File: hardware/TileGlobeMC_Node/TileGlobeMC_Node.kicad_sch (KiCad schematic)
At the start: 112 parts, among them J1 Conn_01x05, J10 LCD, J11 USB_C, J2 P_Male, J3 Conn_01x05, J4 P_Male, J5 Conn_01x05, J6 P_Male, J7 Conn_01x05, J8 P_Male, J9 SWD, Q1 2N7002, Q2 2N7002, SW1 Left, SW2 Left, SW3 Left, SW4 Left, SW5 Left, U1 RP2350_80QFN, U2 TPS62A01DRL, U3 BQ24232RGT, U4 ESP-PSRAM64H, U5 PY25Q128HA-WXH, U6 PY25Q128HA-SSH, U7 74AHC1G04, U8 SC7A20, Y1 12M

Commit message: PCB progress
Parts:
- removed BT1: LIR2032, symbol Device:Battery_Cell
- removed C1, C12, C2, C27, C3, C4, C5, C6, C7, C9: 4.7u, Capacitor_SMD:C_0402_1005Metric, symbol Device:C_Small
- removed C10, C11, C13, C14, C15, C16, C17, C18, C19, C20, C21, C22, C25, C26, C28, C29, C30, C31, C32, C33, C34: 100n, Capacitor_SMD:C_0402_1005Metric, symbol Device:C_Small
- removed C23, C24: 15p, Capacitor_SMD:C_0402_1005Metric, symbol Device:C_Small
- removed C8: 22u, Capacitor_SMD:C_0603_1608Metric, symbol Device:C_Small
- removed D1, D2, D4: 1N4148WT, Diode_SMD:D_SOD-523, symbol Diode:1N4148WT
- removed D3, D5: 3V, Diode_SMD:D_SOD-523, symbol Device:D_Zener_Small
- removed J1, J3, J5, J7: Conn_01x05, symbol Connector_Generic:Conn_01x05
- removed J10: LCD, Connector_FFC-FPC:TE_1-1734839-2_1x12-1MP_P0.5mm_Horizontal, symbol Connector_Generic_MountingPin:Conn_01x12_MountingPin
- removed J11: USB_C, Connector_USB:USB_C_Receptacle_GCT_USB4105-xx-A_16P_TopMnt_Horizontal, symbol Connector:USB_C_Receptacle_USB2.0_16P
- removed J2, J4, J6, J8: P_Male, Project:BC-15-5P380, symbol Connector_Generic_MountingPin:Conn_01x05_MountingPin
- removed J9: SWD, Connector_JST:JST_SH_BM03B-SRSS-TB_1x03-1MP_P1.00mm_Vertical, symbol Connector_Generic_MountingPin:Conn_01x03_MountingPin
- removed JP1: RESET, TestPoint:TestPoint_2Pads_Pitch2.54mm_Drill0.8mm, symbol Jumper:Jumper_2_Small_Open
- removed JP2: USB_BOOT, TestPoint:TestPoint_2Pads_Pitch2.54mm_Drill0.8mm, symbol Jumper:Jumper_2_Small_Open
- removed L1: 3.3u, RP2350:L_pol_2016, symbol Project:L_Polarized_Ferrite_Small
- removed L2: 1u, Inductor_SMD:L_Wuerth_MAPI-2010, symbol Device:L_Ferrite_Small
- removed Q1, Q2: 2N7002, Package_TO_SOT_SMD:SOT-23, symbol Transistor_FET:2N7002
- removed R1, R10, R4, R7: 300, Capacitor_SMD:C_0402_1005Metric, symbol Device:R_Small
- removed R11, R12, R2, R3, R5, R6, R8, R9: 270, Capacitor_SMD:C_0402_1005Metric, symbol Device:R_Small
- removed R13, R24: 33, Capacitor_SMD:C_0402_1005Metric, symbol Device:R_Small
- removed R14, R35, R36, R37, R38, R39, R40, R41: 10k, Capacitor_SMD:C_0402_1005Metric, symbol Device:R_Small
- removed R15: 17.4k, Capacitor_SMD:C_0402_1005Metric, symbol Device:R_Small
- removed R16: 1.5k, Capacitor_SMD:C_0402_1005Metric, symbol Device:R_Small
- removed R17, R18, R19, R22, R23, R28, R29, R34: 100k, Capacitor_SMD:C_0402_1005Metric, symbol Device:R_Small
- removed R20: 86.6k, Capacitor_SMD:C_0402_1005Metric, symbol Device:R_Small
- removed R21: 390k, Capacitor_SMD:C_0402_1005Metric, symbol Device:R_Small
- removed R25, R30: 1k, Capacitor_SMD:C_0402_1005Metric, symbol Device:R_Small
- removed R26, R27: 27, Capacitor_SMD:C_0402_1005Metric, symbol Device:R_Small
- removed R31: 4.7, Capacitor_SMD:C_0402_1005Metric, symbol Device:R_Small
- removed R32, R33: 5.1k, Capacitor_SMD:C_0402_1005Metric, symbol Device:R_Small
- removed SW1, SW2, SW3, SW4, SW5: Left, Button_Switch_SMD:SW_SPST_PTS647_Sx38, symbol Switch:SW_Push
- removed U1: RP2350_80QFN, RP2350:RP2350-QFN-80-1EP_10x10_P0.4mm_EP3.4x3.4mm_ThermalVias, symbol RP2350:RP2350_80QFN
- removed U2: TPS62A01DRL, Package_TO_SOT_SMD:SOT-563, symbol Regulator_Switching:TPS62A01DRL
- removed U3: BQ24232RGT, Package_DFN_QFN:VQFN-16-1EP_3x3mm_P0.5mm_EP1.68x1.68mm_ThermalVias, symbol Project:BQ24232RGT
- removed U4: ESP-PSRAM64H, Package_SO:SOIC-8_3.9x4.9mm_P1.27mm, symbol Project:ESP-PSRAM64
- removed U5: PY25Q128HA-WXH, Package_SON:WSON-8-1EP_6x5mm_P1.27mm_EP3.4x4.3mm, symbol Memory_Flash:W25Q128JVP
- removed U6: PY25Q128HA-SSH, Package_SO:SOIC-8_5.3x5.3mm_P1.27mm, symbol Memory_Flash:W25Q128JVS
- removed U7: 74AHC1G04, Package_TO_SOT_SMD:SOT-23-5, symbol 74xGxx:74AHC1G04
- removed U8: SC7A20, Package_LGA:LGA-12_2x2mm_P0.5mm, symbol Sensor_Motion:SC7A20
- removed Y1: 12M, Crystal:Crystal_SMD_3225-4Pin_3.2x2.5mm, symbol Device:Crystal_GND24
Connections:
- no-connect marks 10 -> 29
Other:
- removed sheet Power
- sheet Core ports: added +3V3, BTN_CENTER, BTN_CENTER_VBUS, GND_CORE, GPIO0, GPIO1, GPIO2, GPIO3, GPIO4, I2C_SCL, I2C_SDA, LCD_CS, LCD_DC, LCD_MOSI, LCD_SCK, PERI_INT, VBUS; removed none
- sheet Peripheral ports: added +3V3, BTN_CENTER, BTN_CENTER_VBUS, GND_PERI, I2C_SCL, I2C_SDA, LCD_CS, LCD_DC, LCD_MOSI, LCD_SCK, PERI_INT, VBUS; removed none
- note removed: "3.3V DC-DC"
- note removed: "Battery Charger & Power Path"
- note removed: "Buttons"
- note removed: "Flash & PSRAM"
- note removed: "IMU"
- note removed: "LCD"
- note removed: "Node Ports"
- note removed: "Note: buttons use MCU's internal pull-down."
- note removed: "TODO: change setting resistors now that we're using bigger batteries"
- note removed: "USB-C"

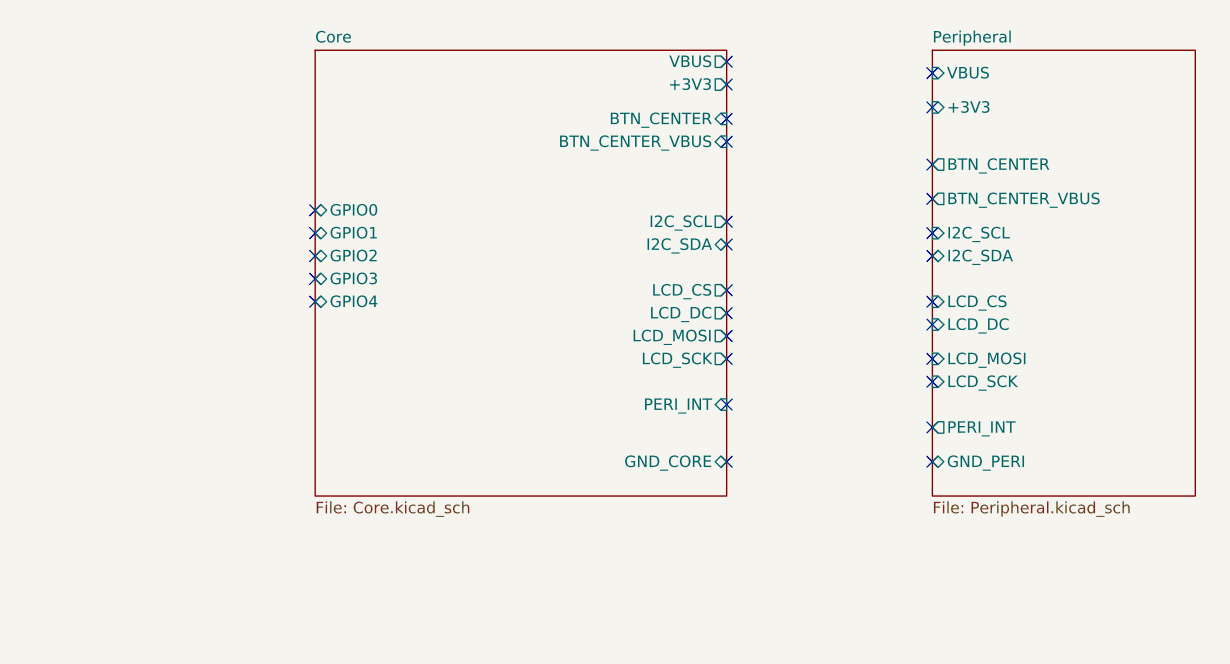
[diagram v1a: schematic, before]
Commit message: PCB progress
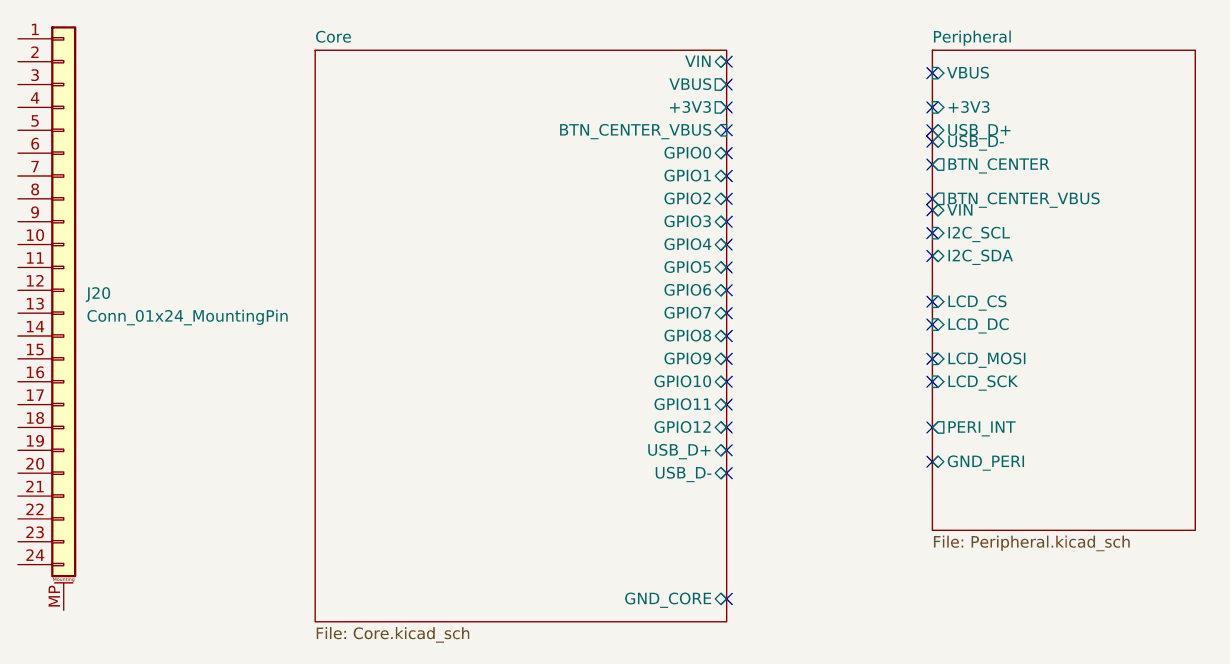
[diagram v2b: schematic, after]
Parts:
- added J20: Conn_01x24_MountingPin, Project:FPC_Verticle_24pin_0.5mm, symbol Connector_Generic_MountingPin:Conn_01x24_MountingPin
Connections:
- no-connect marks 29 -> 35
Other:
- sheet Core ports: added GPIO10, GPIO11, GPIO12, GPIO5, GPIO6, GPIO7, GPIO8, GPIO9, USB_D+, USB_D-, VIN; removed BTN_CENTER, I2C_SCL, I2C_SDA, LCD_CS, LCD_DC, LCD_MOSI, LCD_SCK, PERI_INT
- sheet Peripheral ports: added USB_D+, USB_D-, VIN; removed none

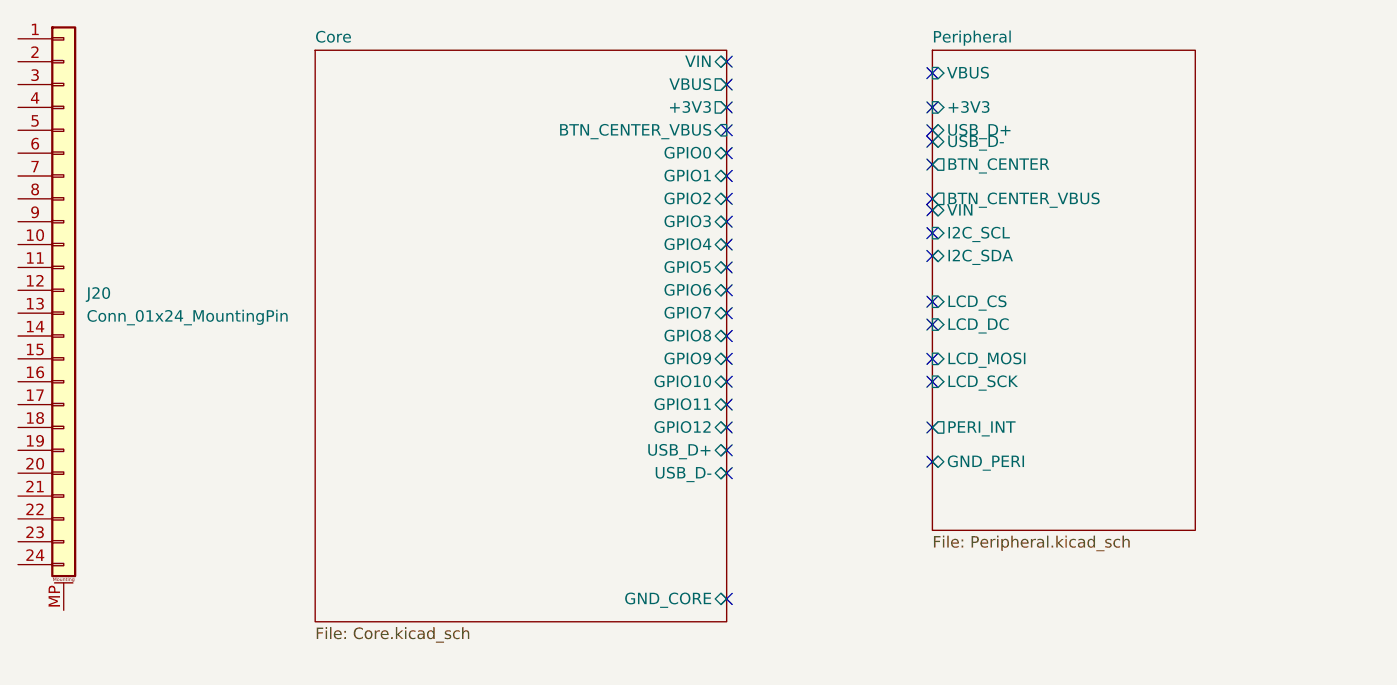
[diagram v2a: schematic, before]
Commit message: Main PCB progress
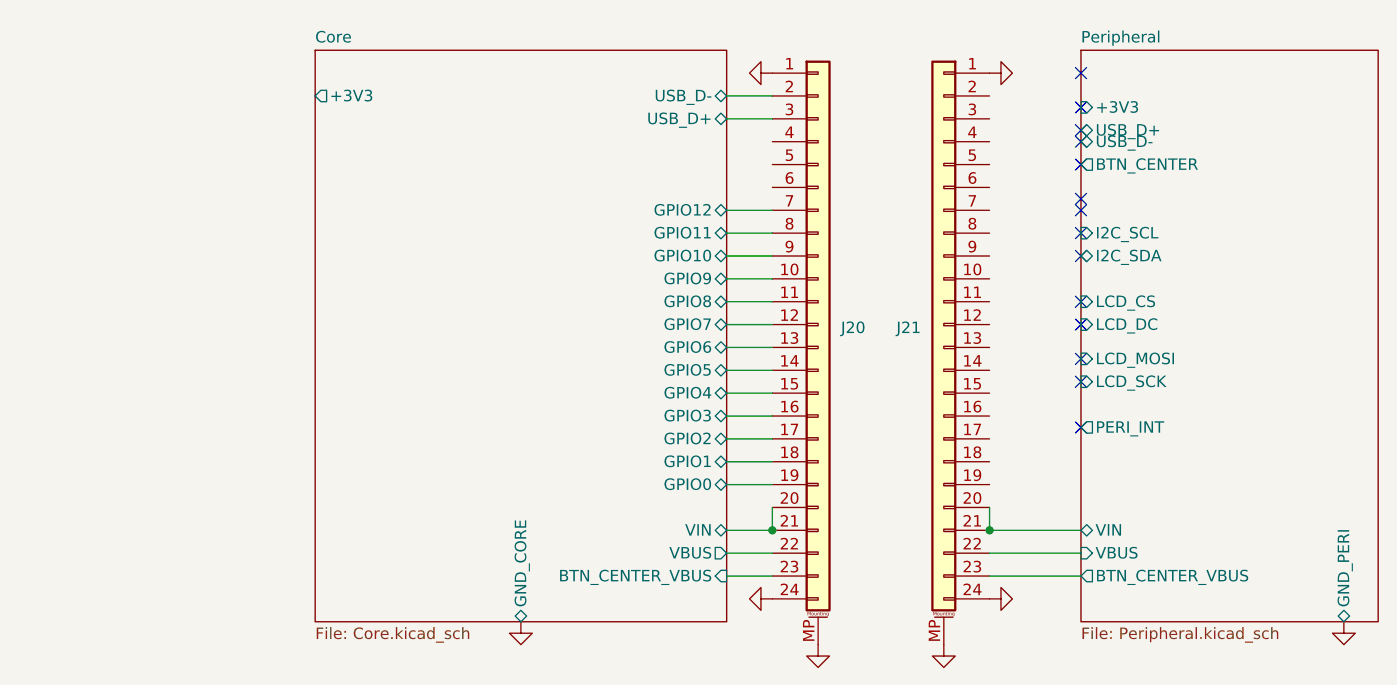
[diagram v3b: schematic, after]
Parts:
- added J21: Conn_01x24_MountingPin, Project:FPC_Verticle_24pin_0.5mm, symbol Connector_Generic_MountingPin:Conn_01x24_MountingPin
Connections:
- net Core/BTN_CENTER_VBUS: now also J20.23 (Pin_23)
- net Core/GPIO0: now also J20.19 (Pin_19)
- net Core/GPIO1: now also J20.18 (Pin_18)
- net Core/GPIO10: now also J20.9 (Pin_9)
- net Core/GPIO11: now also J20.8 (Pin_8)
- net Core/GPIO12: now also J20.7 (Pin_7)
- net Core/GPIO2: now also J20.17 (Pin_17)
- net Core/GPIO3: now also J20.16 (Pin_16)
- net Core/GPIO4: now also J20.15 (Pin_15)
- net Core/GPIO5: now also J20.14 (Pin_14)
- net Core/GPIO6: now also J20.13 (Pin_13)
- net Core/GPIO7: now also J20.12 (Pin_12)
- net Core/GPIO8: now also J20.11 (Pin_11)
- net Core/GPIO9: now also J20.10 (Pin_10)
- net Core/USB_D+: now also J20.3 (Pin_3)
- net Core/USB_D-: now also J20.2 (Pin_2)
- net Core/VBUS: now also J20.22 (Pin_22)
- net Core/VIN: now also J20.20 (Pin_20), J20.21 (Pin_21)
- net Peripheral/BTN_CENTER_VBUS: now also J21.23 (Pin_23)
- net Peripheral/VBUS: now also J21.22 (Pin_22)
- net Peripheral/VIN: now also J21.20 (Pin_20), J21.21 (Pin_21)
- net GND_CORE: now reaches J20.1 (Pin_1)
- net GND_CORE: now also J20.24 (Pin_24), J20.MP (MountPin)
- new net GND_PERI: J21.1 (Pin_1), J21.24 (Pin_24), J21.MP (MountPin)
- no-connect marks 35 -> 14
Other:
- moved on the sheet: J20
